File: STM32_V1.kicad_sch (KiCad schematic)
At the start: 3 parts, among them U1 AMS1117-3.3, U2 STM32F411CEUx, U3 MPU-6050

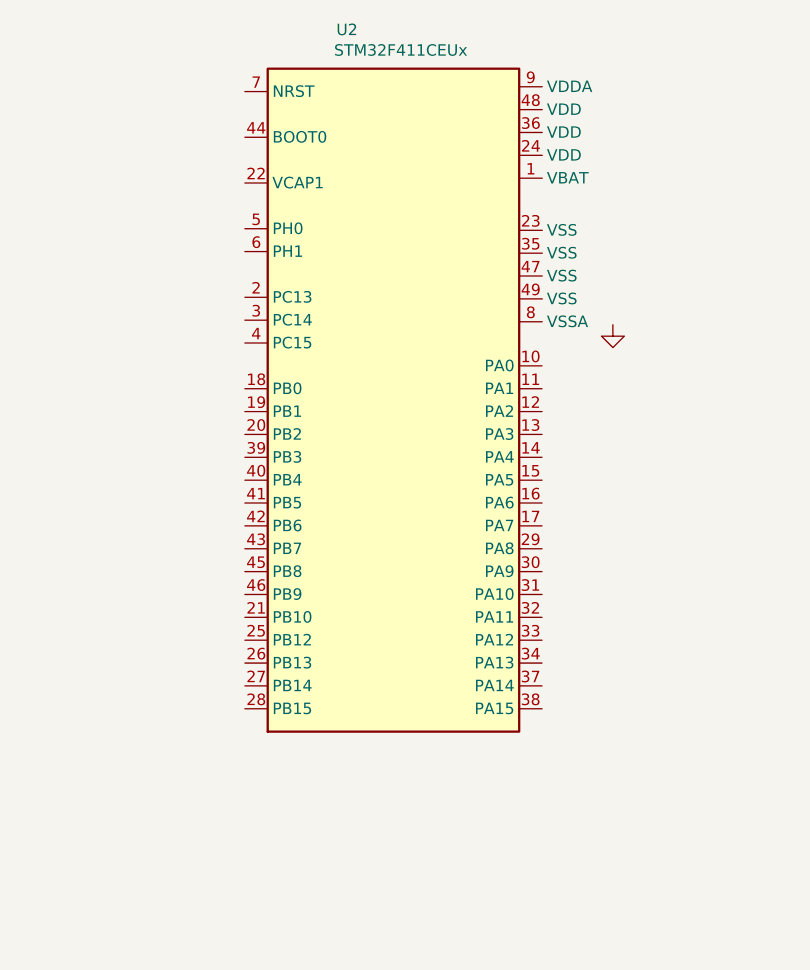
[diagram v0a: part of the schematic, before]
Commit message: 5530
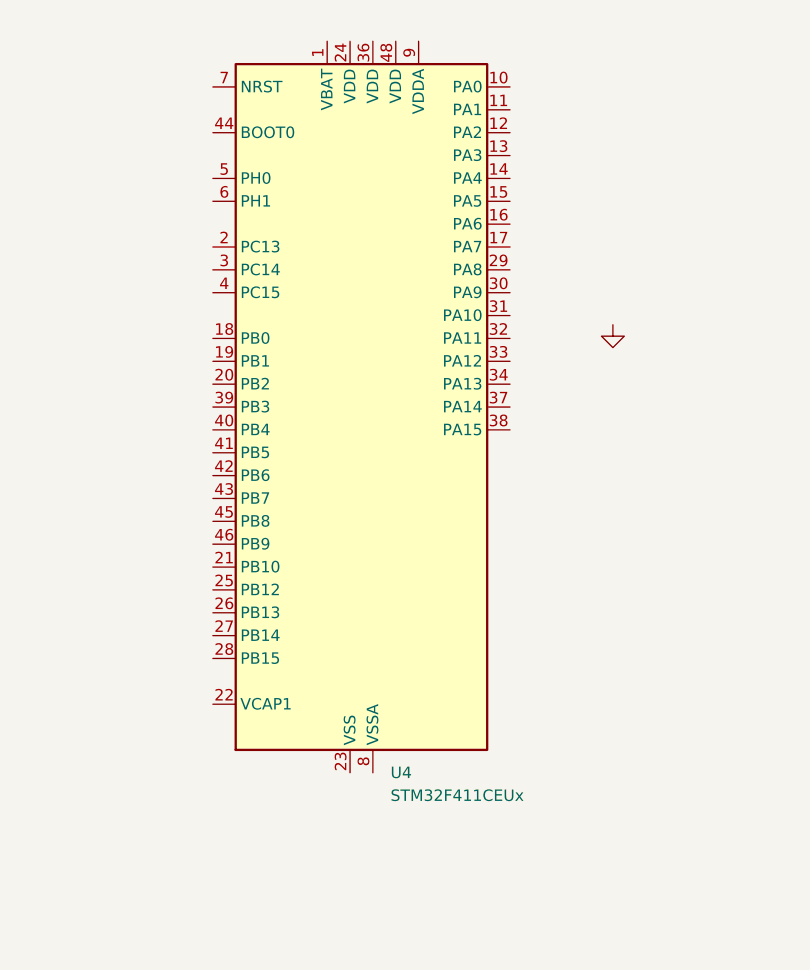
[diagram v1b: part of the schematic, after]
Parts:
- removed U2: STM32F411CEUx, Package_DFN_QFN:QFN-48-1EP_7x7mm_P0.5mm_EP5.6x5.6mm, symbol MCU_ST_STM32F4:STM32F411CEUx
- added U4: STM32F411CEUx, Package_DFN_QFN:QFN-48-1EP_7x7mm_P0.5mm_EP5.6x5.6mm, symbol MCU_ST_STM32F4:STM32F411CEUx
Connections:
- new net: U4.23 (VSS), U4.35 (VSS), U4.47 (VSS), U4.49 (VSS)
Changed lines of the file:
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@@
     )
   )
-  (symbol (lib_id "MCU_ST_STM32F4:STM32F411CEUx") (at 177.546 102.108 0) (unit 1)
-    (in_bom yes) (on_board yes) (dnp no)
-    (property "Reference" "U2" (at 169.926 62.23 0)
+  (symbol (lib_name "STM32F411CEUx_1") (lib_id "MCU_ST_STM32F4:STM32F411CEUx") (at 171.45 104.14 0) (unit 1)
+    (in_bom yes) (on_board yes) (dnp no) (fields_autoplaced)
+    (property "Reference" "U4" (at 175.9459 144.78 0)
       (effects (font (size 1.27 1.27)) (justify left))
     )
-    (property "Value" "STM32F411CEUx" (at 169.672 64.516 0)
+    (property "Value" "STM32F411CEUx" (at 175.9459 147.32 0)
       (effects (font (size 1.27 1.27)) (justify left))
     )
-    (property "Footprint" "Package_DFN_QFN:QFN-48-1EP_7x7mm_P0.5mm_EP5.6x5.6mm" (at 162.306 140.208 0)
+    (property "Footprint" "Package_DFN_QFN:QFN-48-1EP_7x7mm_P0.5mm_EP5.6x5.6mm" (at 158.75 142.24 0)
       (effects (font (size 1.27 1.27)) (justify right) hide)
     )
-    (property "Datasheet" "http://www.st.com/st-web-ui/static/active/en/resource/technical/document/datasheet/DM00115249.pdf" (at 177.546 102.108 0)
+    (property "Datasheet" "https://www.st.com/resource/en/datasheet/stm32f411ce.pdf" (at 171.45 104.14 0)
       (effects (font (size 1.27 1.27)) hide)
     )
@@
       (project "STM32_V1"
         (path "/40d14a59-6a76-4def-8917-b437f2db8c74"
-          (reference "U2") (unit 1)
+          (reference "U4") (unit 1)
         )
       )
